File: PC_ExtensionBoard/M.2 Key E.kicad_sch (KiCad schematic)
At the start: 18 parts, among them J100 Bus_M.2_2199230-2, U2 10GHz

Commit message: update LCSC Number
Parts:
- R132, R133: LCSC (none) -> C242160
- R134, R137: Author Antmicro -> (none); Current 1A -> (none); LCSC (none) -> C242160; License Apache-2.0 -> (none); Manufacturer Panasonic -> (none); Public False -> (none)
- U2: LCSC (none) -> C7498154
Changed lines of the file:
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@@
 			)
 		)
-		(property "Tolerance" ""
-			(at 147.32 77.47 0)
-			(hide yes)
-			(show_name no)
-			(do_not_autoplace no)
-			(effects
-				(font
-					(size 1.27 1.27)
-				)
-				(justify left bottom)
-			)
-		)
-		(property "Current" "1A"
-			(at 129.54 63.5 0)
-			(hide yes)
-			(show_name no)
-			(do_not_autoplace no)
-			(effects
-				(font
-					(size 1.27 1.27)
-					(thickness 0.15)
-				)
-			)
-		)
-		(property "Manufacturer" "Panasonic"
-			(at 147.32 90.17 0)
-			(hide yes)
-			(show_name no)
-			(do_not_autoplace no)
-			(effects
-				(font
-					(size 1.27 1.27)
-					(thickness 0.15)
-				)
-				(justify left bottom)
-			)
-		)
-		(property "License" "Apache-2.0"
-			(at 147.32 92.71 0)
-			(hide yes)
-			(show_name no)
-			(do_not_autoplace no)
-			(effects
-				(font
-					(size 1.27 1.27)
-					(thickness 0.15)
-				)
-				(justify left bottom)
-			)
-		)
-		(property "Author" "Antmicro"
-			(at 147.32 95.25 0)
-			(hide yes)
-			(show_name no)
-			(do_not_autoplace no)
-			(effects
-				(font
-					(size 1.27 1.27)
-					(thickness 0.15)
-				)
-				(justify left bottom)
-			)
-		)
-		(property "Public" "False"
-			(at 147.32 97.79 0)
-			(hide yes)
-			(show_name no)
-			(do_not_autoplace no)
-			(effects
-				(font
-					(size 1.27 1.27)
-				)
-				(justify left bottom)
+		(property "LCSC" "C242160"
+			(at 127 67.31 0)
+			(hide yes)
+			(show_name no)
+			(do_not_autoplace no)
+			(effects
+				(font
+					(size 1.27 1.27)
+				)
 			)
 		)
@@
 			)
 		)
-		(property "Tolerance" ""
-			(at 80.01 146.05 0)
-			(hide yes)
-			(show_name no)
-			(do_not_autoplace no)
-			(effects
-				(font
-					(size 1.27 1.27)
-				)
-				(justify left bottom)
-			)
-		)
-		(property "Current" "1A"
-			(at 62.23 132.715 0)
-			(hide yes)
-			(show_name no)
-			(do_not_autoplace no)
-			(effects
-				(font
-					(size 1.27 1.27)
-					(thickness 0.15)
-				)
-			)
-		)
-		(property "Manufacturer" "Panasonic"
-			(at 80.01 158.75 0)
-			(hide yes)
-			(show_name no)
-			(do_not_autoplace no)
-			(effects
-				(font
-					(size 1.27 1.27)
-					(thickness 0.15)
-				)
-				(justify left bottom)
-			)
-		)
-		(property "License" "Apache-2.0"
-			(at 80.01 161.29 0)
-			(hide yes)
-			(show_name no)
-			(do_not_autoplace no)
-			(effects
-				(font
-					(size 1.27 1.27)
-					(thickness 0.15)
-				)
-				(justify left bottom)
-			)
-		)
-		(property "Author" "Antmicro"
-			(at 80.01 163.83 0)
-			(hide yes)
-			(show_name no)
-			(do_not_autoplace no)
-			(effects
-				(font
-					(size 1.27 1.27)
-					(thickness 0.15)
-				)
-				(justify left bottom)
-			)
-		)
-		(property "Public" "False"
-			(at 80.01 166.37 0)
-			(hide yes)
-			(show_name no)
-			(do_not_autoplace no)
-			(effects
-				(font
-					(size 1.27 1.27)
-				)
-				(justify left bottom)
+		(property "LCSC" "C242160"
+			(at 59.69 135.89 0)
+			(hide yes)
+			(show_name no)
+			(do_not_autoplace no)
+			(effects
+				(font
+					(size 1.27 1.27)
+				)
 			)
 		)
@@
 				)
 				(justify left bottom)
+			)
+		)
+		(property "LCSC" "C242160"
+			(at 49.53 54.61 0)
+			(hide yes)
+			(show_name no)
+			(do_not_autoplace no)
+			(effects
+				(font
+					(size 1.27 1.27)
+				)
 			)
 		)
@@
 			)
 		)
+		(property "LCSC" "C7498154"
+			(at 274.32 35.56 0)
+			(hide yes)
+			(show_name no)
+			(do_not_autoplace no)
+			(effects
+				(font
+					(size 1.27 1.27)
+				)
+			)
+		)
 		(pin "2"
 		)
@@
 			)
 		)
+		(property "LCSC" "C242160"
+			(at 59.69 133.35 0)
+			(hide yes)
+			(show_name no)
+			(do_not_autoplace no)
+			(effects
+				(font
+					(size 1.27 1.27)
+				)
+			)
+		)

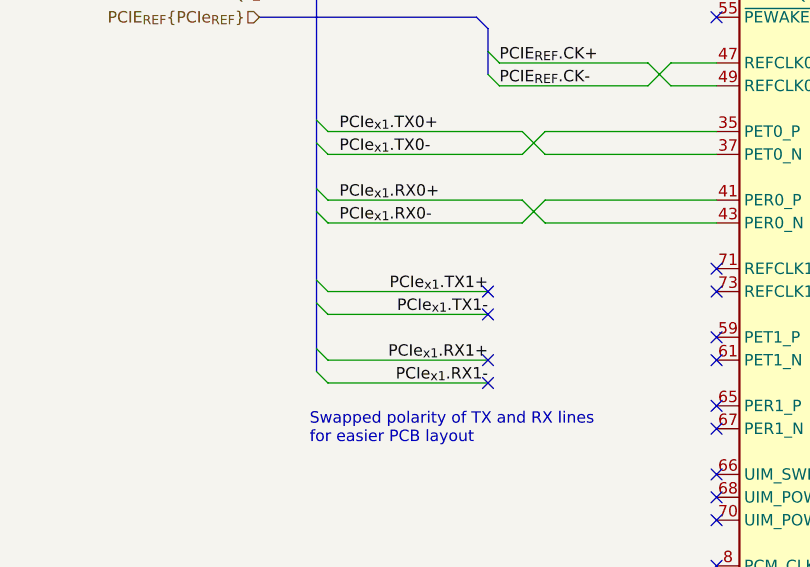
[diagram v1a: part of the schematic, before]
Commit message: update Schematic
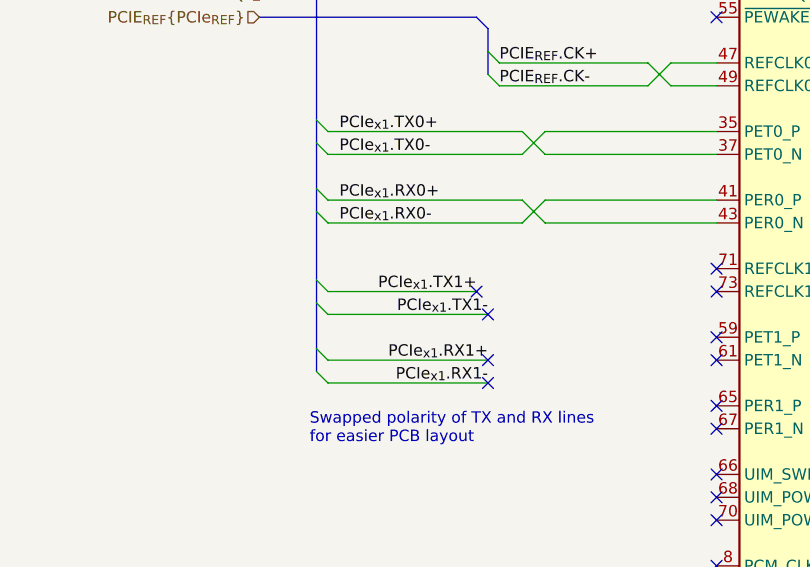
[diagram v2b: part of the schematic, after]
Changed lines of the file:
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@@
+	)
+	(no_connect
+		(at 62.23 92.71)
 	)
 	(no_connect
@@
 	)
 	(no_connect
+		(at 62.23 97.79)
+	)
+	(no_connect
+		(at 62.23 100.33)
+	)
+	(no_connect
 		(at 87.63 95.25)
 	)
@@
 	)
 	(no_connect
-		(at 62.23 100.33)
-	)
-	(no_connect
-		(at 62.23 97.79)
-	)
-	(no_connect
 		(at 118.11 97.79)
 	)
@@
 	)
 	(no_connect
+		(at 60.96 90.17)
+	)
+	(no_connect
 		(at 87.63 140.97)
 	)
@@
 	)
 	(no_connect
-		(at 62.23 90.17)
-	)
-	(no_connect
 		(at 118.11 123.19)
 	)
@@
 	(no_connect
 		(at 118.11 102.87)
-	)
-	(no_connect
-		(at 62.23 92.71)
 	)
 	(no_connect
@@
 	(wire
 		(pts
-			(xy 62.23 90.17) (xy 44.45 90.17)
+			(xy 60.96 90.17) (xy 44.45 90.17)
 		)
 		(stroke
@@
 	)
 	(label "PCIe_{x1}.TX1+"
-		(at 62.23 90.17 180)
+		(at 60.96 90.17 180)
 		(effects
 			(font
